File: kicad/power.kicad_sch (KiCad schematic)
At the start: 106 parts, among them J1 12 V in (5.5x2.1), J2 TX power (shunt), U1 TPS54302DDCR, U2 TPS65131RGER, U3 TPS7A4700RGWT, U4 TPS7A3301RGWR, U5 LM2731XMF, U6 TLV75733PDBVR, U7 TPS7A4700RGWT

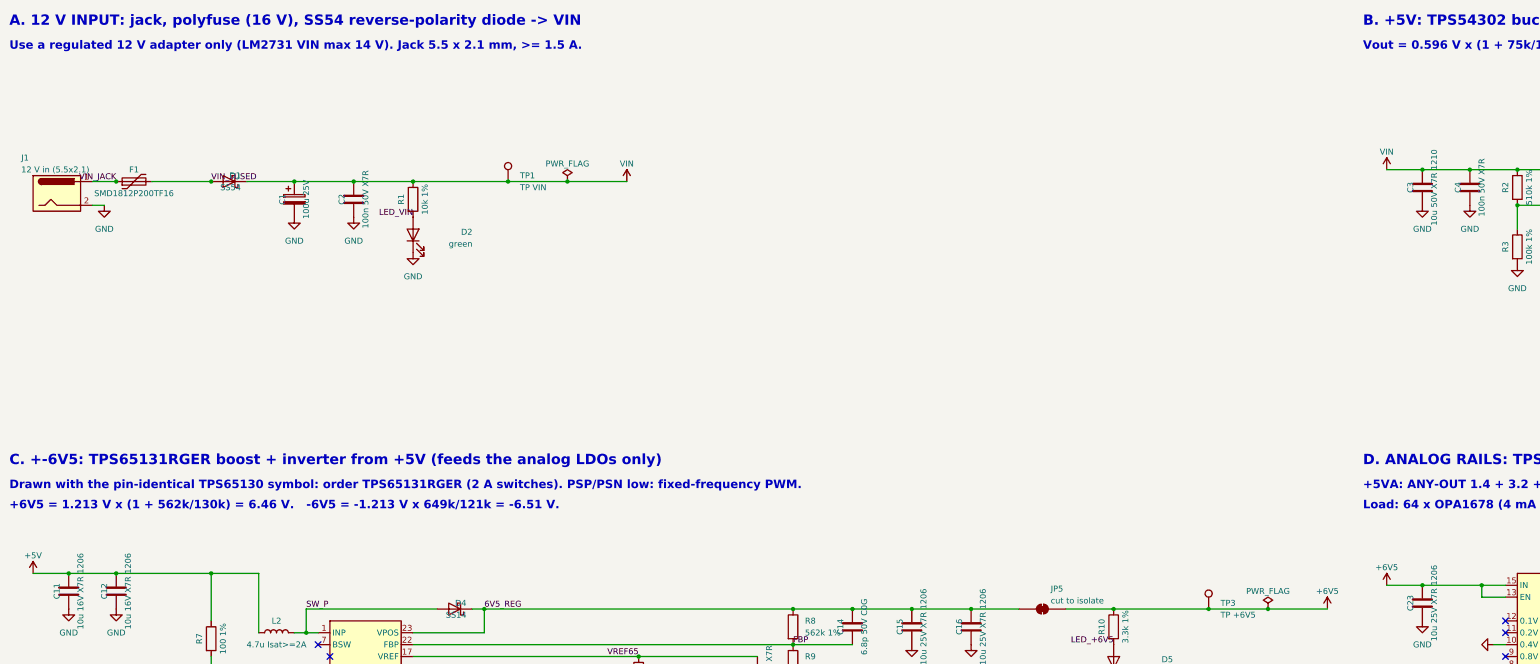
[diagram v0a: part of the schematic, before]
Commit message: Board placement ready for routing; TPS26600 eFuse input protection
PCB (scripts/place.py builds kicad/aesa.kicad_pcb from the schematic, block by block):
- 192 x 301 mm, 4 layers (F.Cu / GND / GND / B.Cu), 3 mm corner bevels, parts >= 3 mm and copper
  >= 0.5 mm from the edge, 6 M3 holes, 3 fiducials
- all cables on the top edge: ribbon headers side by side in the middle, 12 V jack + eFuse top-left,
  +3V3A/+3V3 LDOs top-right; ADC blocks below; array; TX blocks; switchers at the bottom
- channels numbered down the columns: TX group k and ADC k sit under/over the column of CH 4k-3..4k,
  DRV lane left and RX lane right of each column on F.Cu (no crossings)
- hand templates from the mirrored pad positions (TX group, ADC, channel TX parts + op-amp, LM2731
  boost core); everything else placed by connectivity (switch loop first, decoupling at its pin)
- 2.5 mm soldering keep-out around transducer pads; silkscreen: block labels, test-point rail names,
  safety notes on the front
- scripts/placement_check.py: decoupling and switch-loop distances (all pass); DRC 0 violations

Schematic: TPS26600 eFuse (60 V / -60 V, off above 13.8 V and below 8.8 V, 1.6 A, auto-retry)
replaces the SS54 diode; polyfuse kept after it as back-up; test points for adapter voltage, input
current and fault. Array sheet grid follows the board's column-major numbering.
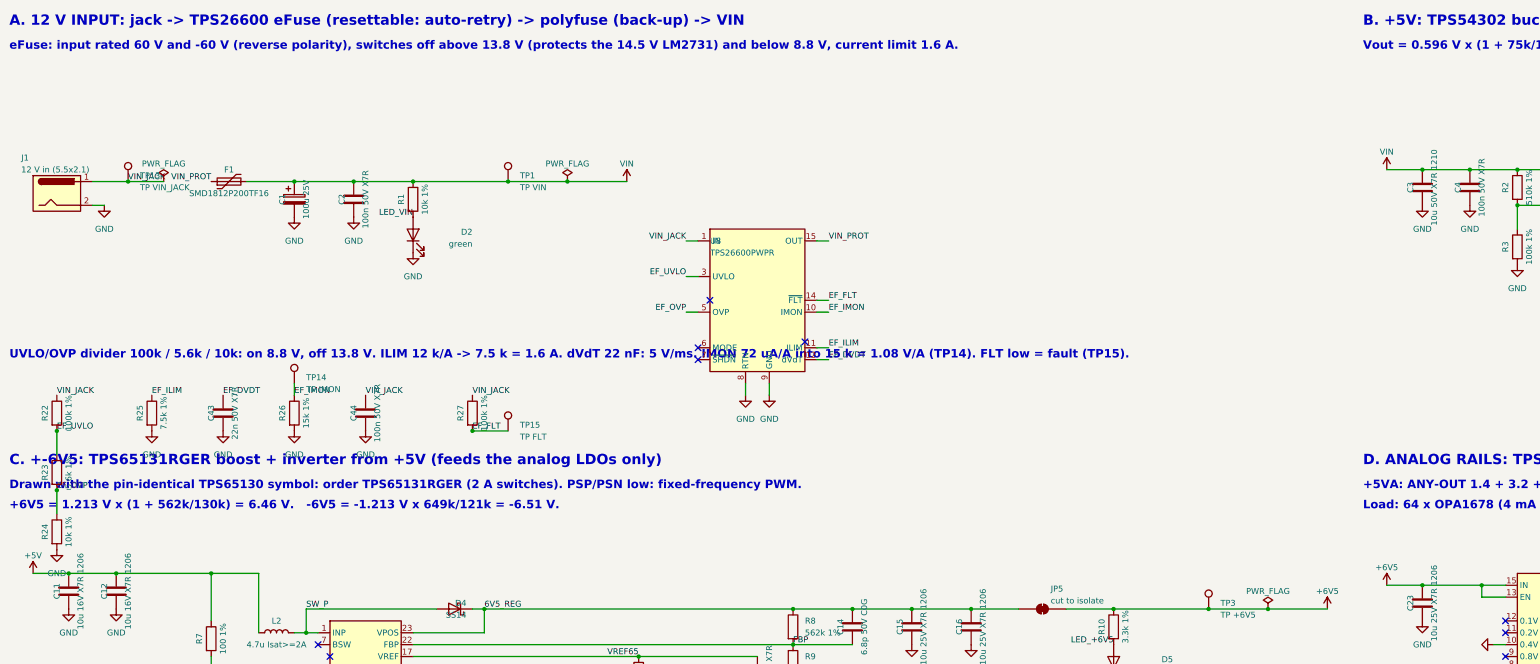
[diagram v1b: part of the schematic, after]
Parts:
- removed D1: SS54, Diode_SMD:D_SMA, symbol Device:D_Schottky
- added C43: 22n 50V X7R, Capacitor_SMD:C_0603_1608Metric, symbol Device:C
- added C44: 100n 50V X7R, Capacitor_SMD:C_0603_1608Metric, symbol Device:C
- added R22, R27: 100k 1%, Resistor_SMD:R_0603_1608Metric, symbol Device:R
- added R23: 5.6k 1%, Resistor_SMD:R_0603_1608Metric, symbol Device:R
- added R24: 10k 1%, Resistor_SMD:R_0603_1608Metric, symbol Device:R
- added R25: 7.5k 1%, Resistor_SMD:R_0603_1608Metric, symbol Device:R
- added R26: 15k 1%, Resistor_SMD:R_0603_1608Metric, symbol Device:R
- added TP13: TP VIN_JACK, TestPoint:TestPoint_Pad_D1.5mm, symbol Connector:TestPoint
- added TP14: TP IMON, TestPoint:TestPoint_Pad_D1.5mm, symbol Connector:TestPoint
- added TP15: TP FLT, TestPoint:TestPoint_Pad_D1.5mm, symbol Connector:TestPoint
- added U8: TPS26600PWPR, Package_SO:HTSSOP-16-1EP_4.4x5mm_P0.65mm_EP3.4x5mm_Mask2.66x2.46mm_ThermalVias, symbol Power_Management:TPS26600PWP
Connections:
- net VIN_FUSED is gone; now on net VIN: F1.2
- net GND: now also C43.2, C44.2, R24.2, R25.2, R26.2, U8.17 (RTN), U8.8 (RTN), U8.9 (GND)
- net VIN_JACK: now also C44.1, R22.1, R27.1, TP13.1, U8.1 (IN), U8.2 (IN); no longer F1.1
- new net EF_DVDT: C43.1, U8.12 (dVdT)
- new net EF_FLT: R27.2, TP15.1, U8.14 (~{FLT})
- new net EF_ILIM: R25.1, U8.11 (ILIM)
- new net EF_IMON: R26.1, TP14.1, U8.10 (IMON)
- new net EF_OVP: R23.2, R24.1, U8.5 (OVP)
- new net EF_UVLO: R22.2, R23.1, U8.3 (UVLO)
- new net VIN_PROT: F1.1, U8.15 (OUT), U8.16 (OUT)
- no-connect marks 15 -> 19
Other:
- note added: "A. 12 V INPUT: jack -> TPS26600 eFuse (resettable: auto-retry) -> polyfuse (back-up) -> VIN"
- note added: "UVLO/OVP divider 100k / 5.6k / 10k: on 8.8 V, off 13.8 V. ILIM 12 k/A -> 7.5 k = 1.6 A. dVdT 22 nF: 5 V/ms. IMON 72 uA/A into 15 k = 1.08 V/A (TP14). FLT low = fault (TP15)."
- note added: "eFuse: input rated 60 V and -60 V (reverse polarity), switches off above 13.8 V (protects the 14.5 V LM2731) and below 8.8 V, current limit 1.6 A."
- note removed: "A. 12 V INPUT: jack, polyfuse (16 V), SS54 reverse-polarity diode -> VIN"
- note removed: "Use a regulated 12 V adapter only (LM2731 VIN max 14 V). Jack 5.5 x 2.1 mm, >= 1.5 A."
